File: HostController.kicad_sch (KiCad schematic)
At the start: 36 parts, among them U1 MX25V5126FZUI, U2 UPD720201K8-7x1-BAC-A, Y1 ECS-240-8-37B-CKY-TR

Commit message: refactor: standardize project structure and link central purdue-rov-kicad-lib
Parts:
- U1: symbol ROV_PCIe_USB_HUB:MX25V5126FZUI -> rov_logic:MX25V5126FZUI
- U2: footprint ROV_PCIe_USB_HUB:QFN-68-1EP_8x8mm_P0.4mm_EP6.2x6.2mm -> rov_logic:QFN-68-1EP_8x8mm_P0.4mm_EP6.2x6.2mm; symbol ROV_PCIe_USB_HUB:UPD720201K8-7x1-BAC-A -> rov_logic:UPD720201K8-7x1-BAC-A

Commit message: readme + board changes
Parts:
- U1: Category (none) -> Logic; DigiKey (none) -> 1092-1065-1-ND; MPN (none) -> MX25V5126FZUI; Manufacturer (none) -> Macronix; Temp_Range (none) -> -40°C to 85°C; Verified (none) -> Yes
- U2: Category (none) -> Logic; DigiKey (none) -> UPD720201K8-711-BAC-ACT-ND; MPN (none) -> UPD720201K8-711-BAC-A; Manufacturer (none) -> Renesas Electronics Corporation; Temp_Range (none) -> 0°C to 85°C; Verified (none) -> Yes
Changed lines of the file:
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@@
 			)
 		)
-		(property "Datasheet" "MX25V5126FZUI"
+		(property "Datasheet" "https://www.macronix.com/Lists/Datasheet/Attachments/7434/MX25V5126F,%202.5V-3.6V,%20512Kb,%20v1.1.pdf"
 			(at 64.262 112.776 0)
 			(hide yes)
@@
 			)
 		)
-		(property "Description" ""
+		(property "Description" "512Kb (64K x 8) Serial NOR Flash Memory, SPI, 8-USON"
 			(at 54.61 104.14 0)
 			(hide yes)
@@
 		)
 		(property "Part Number" "MX25V5126FZUI"
+			(at 54.61 104.14 0)
+			(hide yes)
+			(show_name no)
+			(do_not_autoplace no)
+			(effects
+				(font
+					(size 1.27 1.27)
+				)
+			)
+		)
+		(property "Manufacturer" "Macronix"
+			(at 54.61 104.14 0)
+			(hide yes)
+			(show_name no)
+			(do_not_autoplace no)
+			(effects
+				(font
+					(size 1.27 1.27)
+				)
+			)
+		)
+		(property "MPN" "MX25V5126FZUI"
+			(at 54.61 104.14 0)
+			(hide yes)
+			(show_name no)
+			(do_not_autoplace no)
+			(effects
+				(font
+					(size 1.27 1.27)
+				)
+			)
+		)
+		(property "DigiKey" "1092-1065-1-ND"
+			(at 54.61 104.14 0)
+			(hide yes)
+			(show_name no)
+			(do_not_autoplace no)
+			(effects
+				(font
+					(size 1.27 1.27)
+				)
+			)
+		)
+		(property "Temp_Range" "-40°C to 85°C"
+			(at 54.61 104.14 0)
+			(hide yes)
+			(show_name no)
+			(do_not_autoplace no)
+			(effects
+				(font
+					(size 1.27 1.27)
+				)
+			)
+		)
+		(property "Category" "Logic"
+			(at 54.61 104.14 0)
+			(hide yes)
+			(show_name no)
+			(do_not_autoplace no)
+			(effects
+				(font
+					(size 1.27 1.27)
+				)
+			)
+		)
+		(property "Verified" "Yes"
 			(at 54.61 104.14 0)
 			(hide yes)
@@
 			)
 		)
-		(property "Datasheet" "UPD720201K8-701-BAC-A"
+		(property "Datasheet" "https://www.renesas.com/en/document/dst/upd720201-upd720202-datasheet.pdf"
 			(at 138.176 148.082 0)
 			(hide yes)
@@
 			)
 		)
-		(property "Description" ""
+		(property "Description" "USB 3.0 Host Controller, 4 Ports, PCIe to USB 3.0, 68-QFN"
 			(at 137.16 55.88 0)
 			(hide yes)
@@
 			(at 162.56 97.79 0)
 			(hide yes)
+			(show_name no)
+			(do_not_autoplace no)
+			(effects
+				(font
+					(size 1.27 1.27)
+				)
+			)
+		)
+		(property "Manufacturer" "Renesas Electronics Corporation"
+			(at 162.56 97.79 0)
+			(hide yes)
+			(show_name no)
+			(do_not_autoplace no)
+			(effects
+				(font
+					(size 1.27 1.27)
+				)
+			)
+		)
+		(property "MPN" "UPD720201K8-711-BAC-A"
+			(at 162.56 97.79 0)
+			(hide yes)
+			(show_name no)
+			(do_not_autoplace no)
+			(effects
+				(font
+					(size 1.27 1.27)
+				)
+			)
+		)
+		(property "DigiKey" "UPD720201K8-711-BAC-ACT-ND"
+			(at 162.56 97.79 0)
+			(hide yes)
+			(show_name no)
+			(do_not_autoplace no)
+			(effects
+				(font
+					(size 1.27 1.27)
+				)
+			)
+		)
+		(property "Temp_Range" "0°C to 85°C"
+			(at 162.56 97.79 0)
+			(hide yes)
+			(show_name no)
+			(do_not_autoplace no)
+			(effects
+				(font
+					(size 1.27 1.27)
+				)
+			)
+		)
+		(property "Category" "Logic"
+			(at 162.56 97.79 0)
+			(hide yes)
+			(show_name no)
+			(do_not_autoplace no)
+			(effects
+				(font
+					(size 1.27 1.27)
+				)
+			)
+		)
+		(property "Verified" "Yes"
+			(at 162.56 97.79 0)
+			(hide yes)

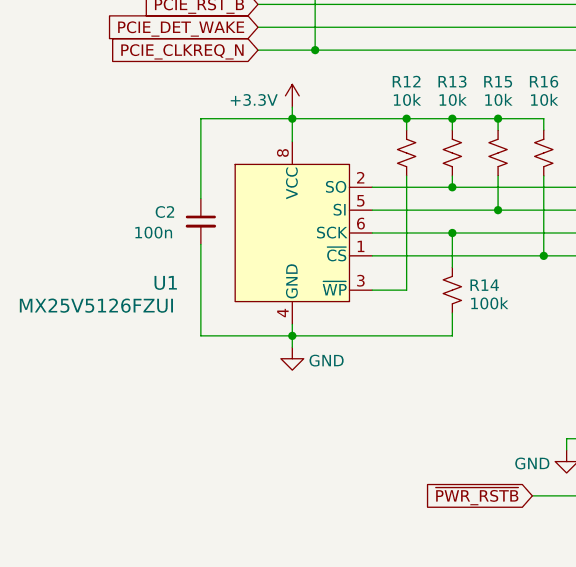
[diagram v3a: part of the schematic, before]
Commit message: updates
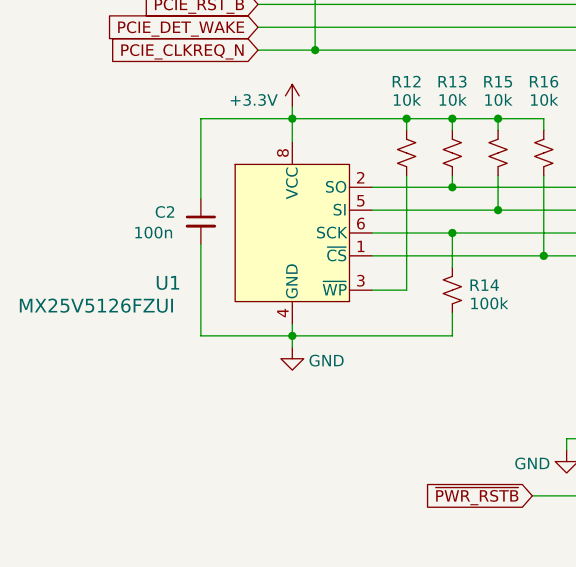
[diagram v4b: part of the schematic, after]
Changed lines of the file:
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@@
 		(dnp no)
 		(property "Reference" "U1"
-			(at 39.116 110.998 0)
+			(at 39.37 110.998 0)
 			(show_name no)
 			(do_not_autoplace no)
